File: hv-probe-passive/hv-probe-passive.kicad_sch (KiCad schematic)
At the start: 20 parts, among them J2 OUT

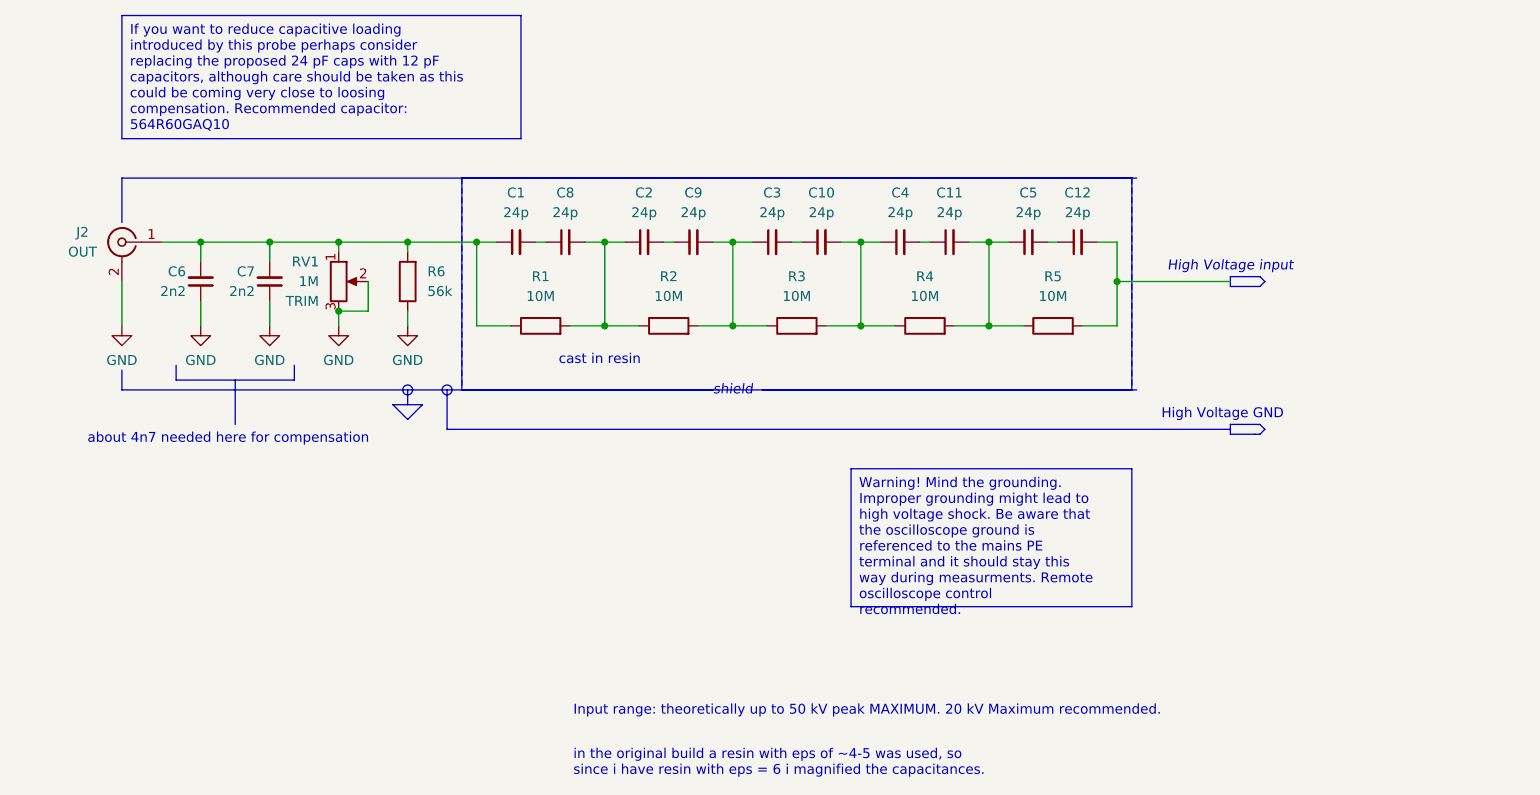
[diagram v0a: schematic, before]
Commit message: cleaned up the schematic and readme
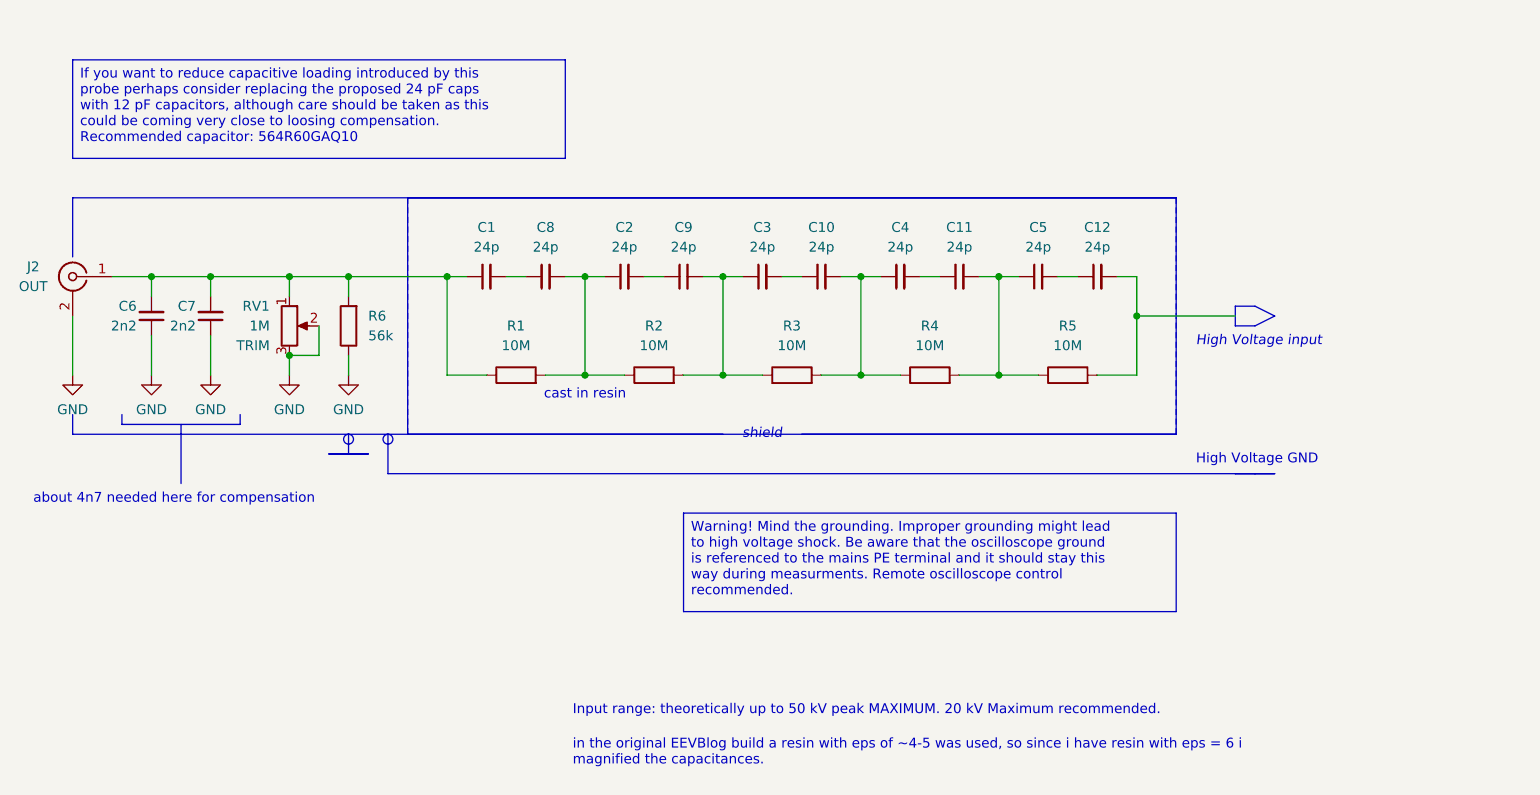
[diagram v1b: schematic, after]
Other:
- moved on the sheet: C1, C10, C11, C12, C2, C3, C4, C5, C6, C7, C8, C9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

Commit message: testing further readme improvements
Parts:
- C6, C7: MPN Nr prod.: VJ1206A222FFBAT -> VJ1206A222FFBAT
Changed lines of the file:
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@@
 			)
 		)
-		(property "MPN" "Nr prod.: VJ1206A222FFBAT"
+		(property "MPN" "VJ1206A222FFBAT"
 			(at 38.1 55.88 0)
 			(hide yes)
@@
 			)
 		)
-		(property "MPN" "Nr prod.: VJ1206A222FFBAT"
+		(property "MPN" "VJ1206A222FFBAT"
 			(at 45.72 55.88 0)
 			(hide yes)
